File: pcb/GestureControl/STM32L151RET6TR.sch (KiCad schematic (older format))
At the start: 41 parts, among them J10 EXTERN I2C, J11 Conn_01x01, J12 Conn_01x01, J13 Conn_01x01, J14 Conn_01x01, J15 Conn_01x01, J16 Conn_01x01, J17 Conn_01x01, J18 Conn_01x01, J19 Conn_01x01, J7 FTDI, J8 Serial Wire, J9 UART, SW3 BOOT, SW4 RST, U6 STM32L151RETx, U7 STM32F401RETx, Y1 8MHz, Y2 32kHz

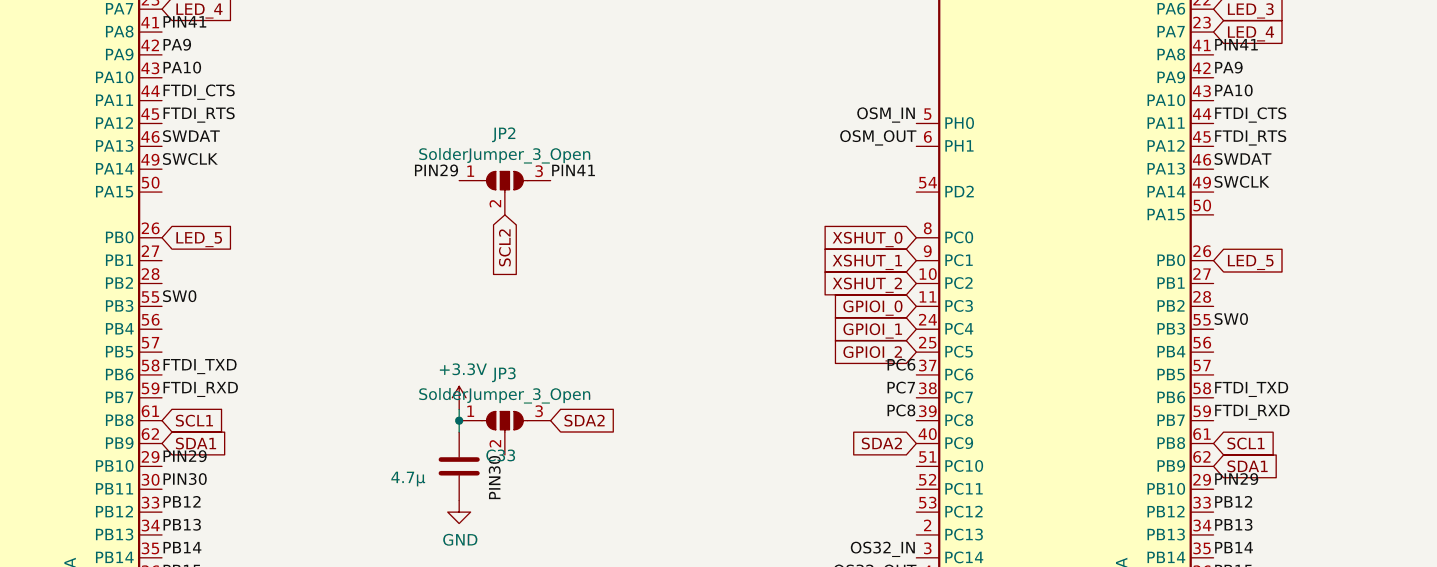
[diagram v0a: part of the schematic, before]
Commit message: eind tekenen PCB
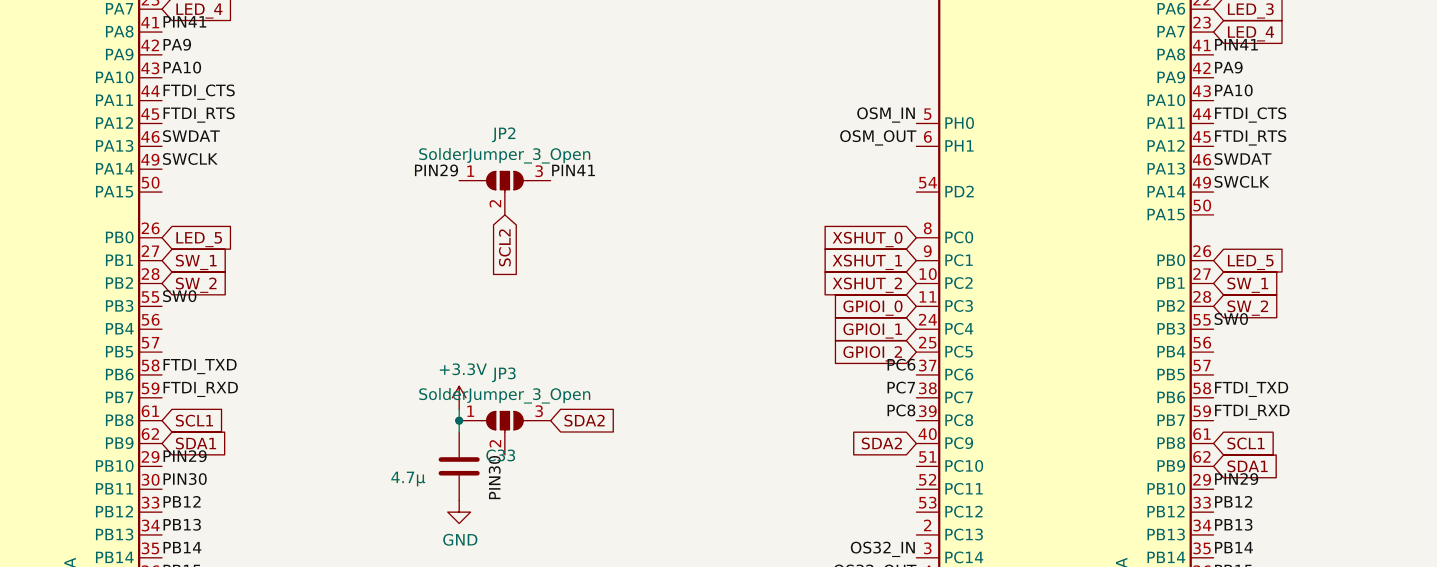
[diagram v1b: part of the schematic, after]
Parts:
- J10: footprint Connector_PinHeader_2.54mm:PinHeader_1x04_P2.54mm_Horizontal -> Connector_PinHeader_2.54mm:PinHeader_1x04_P2.54mm_Vertical
- J7: footprint Connector_PinHeader_2.54mm:PinHeader_1x06_P2.54mm_Horizontal -> Connector_PinHeader_2.54mm:PinHeader_1x06_P2.54mm_Vertical
- J8: footprint Connector_PinHeader_2.54mm:PinHeader_1x05_P2.54mm_Horizontal -> Connector_PinHeader_2.54mm:PinHeader_1x05_P2.54mm_Vertical
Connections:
- net labels added: SW_1, SW_2
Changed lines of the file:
@@
 Wire Wire Line
 	1950 2750 1700 2750
-$Comp
-L Device:C C21
-U 1 1 623C6A21
-P 2150 3050
-AR Path="/623BE0FF/623C6A21" Ref="C21"  Part="1"
-AR Path="/623BC61F/623C6A21" Ref="C?"  Part="1"
-F 0 "C21" V 1898 3050 50  0000 C CNN
-F 1 "100n" V 1989 3050 50  0000 C CNN
-F 2 "Capacitor_SMD:C_0603_1608Metric_Pad1.08x0.95mm_HandSolder" H 2188 2900 50  0001 C CNN
-F 3 "~" H 2150 3050 50  0001 C CNN
-	1    2150 3050
-	0    1    1    0
-$EndComp
 Wire Wire Line
 	1700 2550 1700 2750
@@
 F 0 "J7" H 7580 992 50  0000 L CNN
 F 1 "FTDI" H 7580 901 50  0000 L CNN
-F 2 "Connector_PinHeader_2.54mm:PinHeader_1x06_P2.54mm_Horizontal" H 7500 1000 50  0001 C CNN
+F 2 "Connector_PinHeader_2.54mm:PinHeader_1x06_P2.54mm_Vertical" H 7500 1000 50  0001 C CNN
 F 3 "~" H 7500 1000 50  0001 C CNN
 	1    7500 1000
@@
 F 0 "J8" H 7580 1842 50  0000 L CNN
 F 1 "Serial Wire" H 7580 1751 50  0000 L CNN
-F 2 "Connector_PinHeader_2.54mm:PinHeader_1x05_P2.54mm_Horizontal" H 7500 1800 50  0001 C CNN
+F 2 "Connector_PinHeader_2.54mm:PinHeader_1x05_P2.54mm_Vertical" H 7500 1800 50  0001 C CNN
 F 3 "~" H 7500 1800 50  0001 C CNN
 	1    7500 1800
@@
 F 0 "J10" H 10580 1092 50  0000 L CNN
 F 1 "EXTERN I2C" H 10580 1001 50  0000 L CNN
-F 2 "Connector_PinHeader_2.54mm:PinHeader_1x04_P2.54mm_Horizontal" H 10500 1100 50  0001 C CNN
+F 2 "Connector_PinHeader_2.54mm:PinHeader_1x04_P2.54mm_Vertical" H 10500 1100 50  0001 C CNN
 F 3 "~" H 10500 1100 50  0001 C CNN
 	1    10500 1100
@@
 	1    0    0    -1
 $EndComp
+$Comp
+L Device:C C21
+U 1 1 623C6A21
+P 2150 3050
+AR Path="/623BE0FF/623C6A21" Ref="C21"  Part="1"
+AR Path="/623BC61F/623C6A21" Ref="C?"  Part="1"
+F 0 "C21" V 1898 3050 50  0000 C CNN
+F 1 "100n" V 1989 3050 50  0000 C CNN
+F 2 "Capacitor_SMD:C_0603_1608Metric_Pad1.08x0.95mm_HandSolder" H 2188 2900 50  0001 C CNN
+F 3 "~" H 2150 3050 50  0001 C CNN
+	1    2150 3050
+	0    1    1    0
+$EndComp
+Text GLabel 5600 4650 2    50   Input ~ 0
+SW_1
+Text GLabel 10200 4850 2    50   Input ~ 0
+SW_2
+Text GLabel 10200 4750 2    50   Input ~ 0
+SW_1
+Text GLabel 5600 4750 2    50   Input ~ 0
+SW_2
 $EndSCHEMATC

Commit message: add feedback Philip
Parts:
- removed J8: Serial Wire, Connector_PinHeader_2.54mm:PinHeader_1x05_P2.54mm_Vertical, symbol Connector_Generic:Conn_01x05
- added J8: Conn_01x06, Connector_PinHeader_2.54mm:PinHeader_1x06_P2.54mm_Vertical, symbol Connector_Generic:Conn_01x06
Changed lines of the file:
@@
 Text Label 7300 1300 2    50   ~ 0
 FTDI_RTS
-Text Label 7300 1800 2    50   ~ 0
-SWDAT
-Text Label 7300 1900 2    50   ~ 0
-SWCLK
 Text Label 2450 3450 2    50   ~ 0
 MCO
@@
 	2450 3450 2450 3750
 Connection ~ 2450 3750
-Text Label 7300 2000 2    50   ~ 0
-SW0
 Text Label 5600 4150 0    50   ~ 0
 SWDAT
@@
 	1    7500 1000
 	1    0    0    -1
-$EndComp
-$Comp
-L Connector_Generic:Conn_01x05 J8
-U 1 1 623C6A0C
-P 7500 1800
-AR Path="/623BE0FF/623C6A0C" Ref="J8"  Part="1"
-AR Path="/623BC61F/623C6A0C" Ref="J?"  Part="1"
-F 0 "J8" H 7580 1842 50  0000 L CNN
-F 1 "Serial Wire" H 7580 1751 50  0000 L CNN
-F 2 "Connector_PinHeader_2.54mm:PinHeader_1x05_P2.54mm_Vertical" H 7500 1800 50  0001 C CNN
-F 3 "~" H 7500 1800 50  0001 C CNN
-	1    7500 1800
-	1    0    0    -1
-$EndComp
-$Comp
-L power:+3.3V #PWR081
-U 1 1 623C6A0D
-P 7300 1700
-AR Path="/623BE0FF/623C6A0D" Ref="#PWR081"  Part="1"
-AR Path="/623BC61F/623C6A0D" Ref="#PWR?"  Part="1"
-F 0 "#PWR081" H 7300 1550 50  0001 C CNN
-F 1 "+3.3V" V 7315 1828 50  0000 L CNN
-F 2 "" H 7300 1700 50  0001 C CNN
-F 3 "" H 7300 1700 50  0001 C CNN
-	1    7300 1700
-	0    -1   -1   0
-$EndComp
-$Comp
-L power:GND #PWR080
-U 1 1 623C6A0E
-P 7300 1600
-AR Path="/623BE0FF/623C6A0E" Ref="#PWR080"  Part="1"
-AR Path="/623BC61F/623C6A0E" Ref="#PWR?"  Part="1"
-F 0 "#PWR080" H 7300 1350 50  0001 C CNN
-F 1 "GND" V 7305 1472 50  0000 R CNN
-F 2 "" H 7300 1600 50  0001 C CNN
-F 3 "" H 7300 1600 50  0001 C CNN
-	1    7300 1600
-	0    1    1    0
 $EndComp
 Text Label 5600 4850 0    50   ~ 0
@@
 Text GLabel 5600 4750 2    50   Input ~ 0
 SW_2
+$Comp
+L Connector_Generic:Conn_01x06 J8
+U 1 1 621F67F1
+P 7500 2550
+F 0 "J8" H 7580 2542 50  0000 L CNN
+F 1 "Conn_01x06" H 7580 2451 50  0000 L CNN
+F 2 "Connector_PinHeader_2.54mm:PinHeader_1x06_P2.54mm_Vertical" H 7500 2550 50  0001 C CNN
+F 3 "~" H 7500 2550 50  0001 C CNN
+	1    7500 2550
+	1    0    0    -1
+$EndComp
+$Comp
+L power:+3.3V #PWR0114
+U 1 1 621F7626
+P 7300 2350
+AR Path="/623BE0FF/621F7626" Ref="#PWR0114"  Part="1"
+AR Path="/623BC61F/621F7626" Ref="#PWR?"  Part="1"
+F 0 "#PWR0114" H 7300 2200 50  0001 C CNN
+F 1 "+3.3V" V 7315 2478 50  0000 L CNN
+F 2 "" H 7300 2350 50  0001 C CNN
+F 3 "" H 7300 2350 50  0001 C CNN
+	1    7300 2350
+	0    -1   -1   0
+$EndComp
+Text Label 7300 2450 2    50   ~ 0
+SWCLK
+$Comp
+L power:GND #PWR0115
+U 1 1 621F7BD3
+P 7300 2550
+AR Path="/623BE0FF/621F7BD3" Ref="#PWR0115"  Part="1"
+AR Path="/623BC61F/621F7BD3" Ref="#PWR?"  Part="1"
+F 0 "#PWR0115" H 7300 2300 50  0001 C CNN
+F 1 "GND" V 7305 2422 50  0000 R CNN
+F 2 "" H 7300 2550 50  0001 C CNN
+F 3 "" H 7300 2550 50  0001 C CNN
+	1    7300 2550
+	0    1    1    0
+$EndComp
+Text Label 7300 2650 2    50   ~ 0
+SWDAT
+Text Label 7300 2750 2    50   ~ 0
+RST
+Text Label 7300 2850 2    50   ~ 0
+SW0
 $EndSCHEMATC

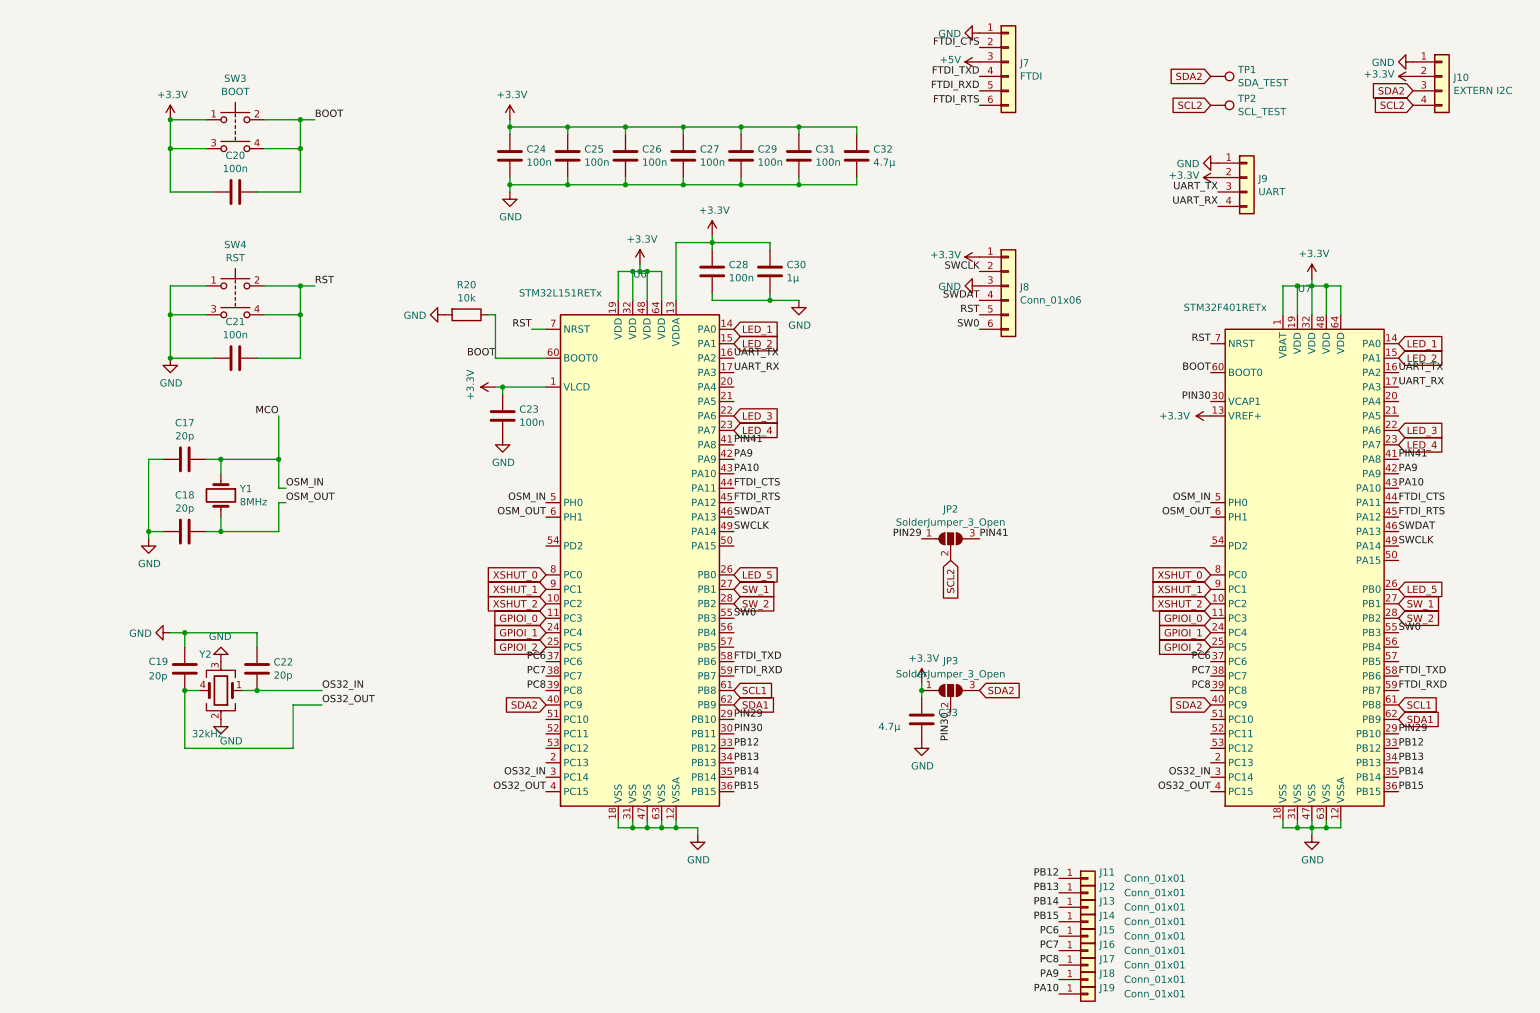
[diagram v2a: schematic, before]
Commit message: werking printf()
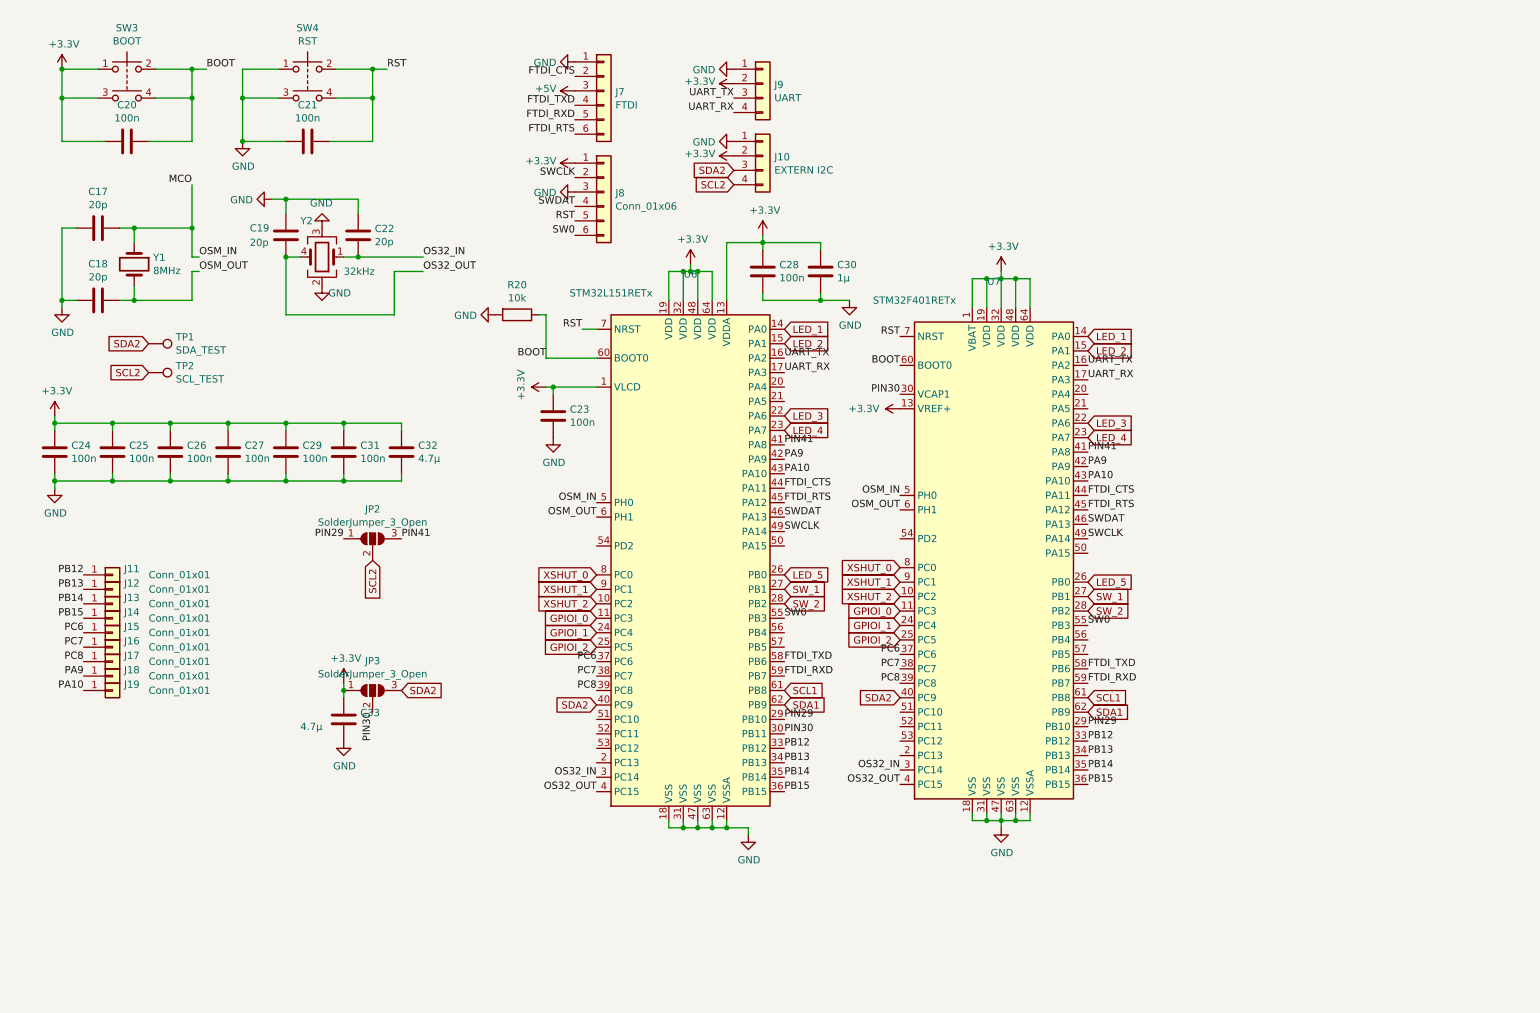
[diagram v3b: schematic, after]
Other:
- moved on the sheet: C17, C18, C19, C20, C21, C22, C23, C24, C25, C26, C27, C28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

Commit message: add PCBV0.11
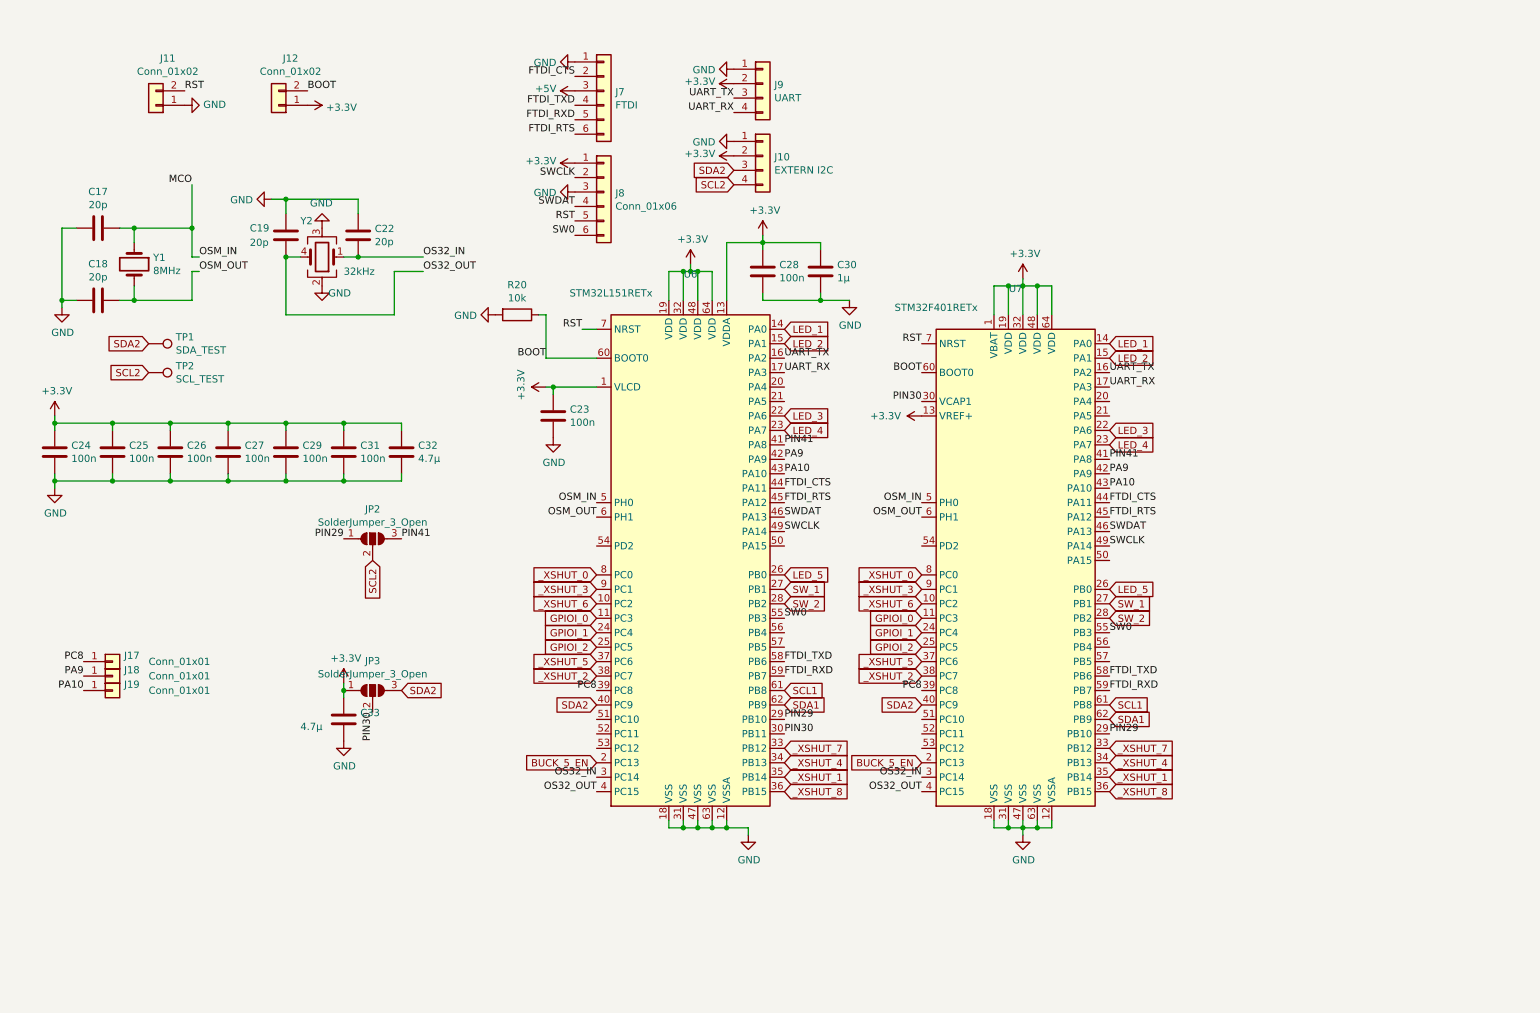
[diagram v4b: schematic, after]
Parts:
- removed C20, C21: 100n, Capacitor_SMD:C_0603_1608Metric_Pad1.08x0.95mm_HandSolder, symbol Device:C
- removed J11, J12, J13, J14, J15, J16: Conn_01x01, TestPoint:TestPoint_Pad_1.5x1.5mm, symbol Connector_Generic:Conn_01x01
- removed SW3: BOOT, Button_Switch_SMD:SW_Push_1P1T_NO_6x6mm_H9.5mm, symbol Switch:SW_Push_Dual
- removed SW4: RST, Button_Switch_SMD:SW_Push_1P1T_NO_6x6mm_H9.5mm, symbol Switch:SW_Push_Dual
- added J11, J12: Conn_01x02, Connector_PinHeader_2.54mm:PinHeader_1x02_P2.54mm_Vertical, symbol Connector_Generic:Conn_01x02
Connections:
- net +3V3: now also J12.1 (Pin_1)
- net BOOT: now also J12.2 (Pin_2)
- net GND: now also J11.1 (Pin_1)
- net RST: now also J11.2 (Pin_2)
- net BUCK_5_EN: now reaches U6.2 (PC13)
- net BUCK_5_EN: now also U7.2 (PC13)
- net PB12 renamed _XSHUT_7
- net PB13 renamed _XSHUT_4
- net PB14 renamed _XSHUT_1
- net PB15 renamed _XSHUT_8
- net PC6 renamed _XSHUT_5
- net PC7 renamed _XSHUT_2
- net XSHUT_0 renamed _XSHUT_0
- net XSHUT_1 renamed _XSHUT_3
- net XSHUT_2 renamed _XSHUT_6
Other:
- moved on the sheet: U7
